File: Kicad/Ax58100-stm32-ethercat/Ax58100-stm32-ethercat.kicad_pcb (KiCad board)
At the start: 2 copper layers, 95.3 x 87.9 mm, 183 parts, among them J1 Step1, J10 5V Power IN, J11 24V Field, J12 DAC, J13 Encoder, J14 In_opt2, J15 STLINK, J16 Serial usart1, J17 In_opt1, J18 Out_opt, J2 Step2, J3 Step3, J4 Step4, J5 THCAD, J6 In1-4, J7 In5-8, J8 Output1-2, J9 Output3-4, SW1 SW PB, U10 AMS1117-1.2, U11 AX58100, U12 TXS0108EPW, U3 MAX3485CSA/ESA, U4 TLP292-4, U5 TLP292-4, U6 TLP292-4, U7 STM32F407VGT6, U8 AMS1117-3.3, U9 24LC32A, Y1 8 MHz, Y2 NXK25.000AE12F-KAB6-12

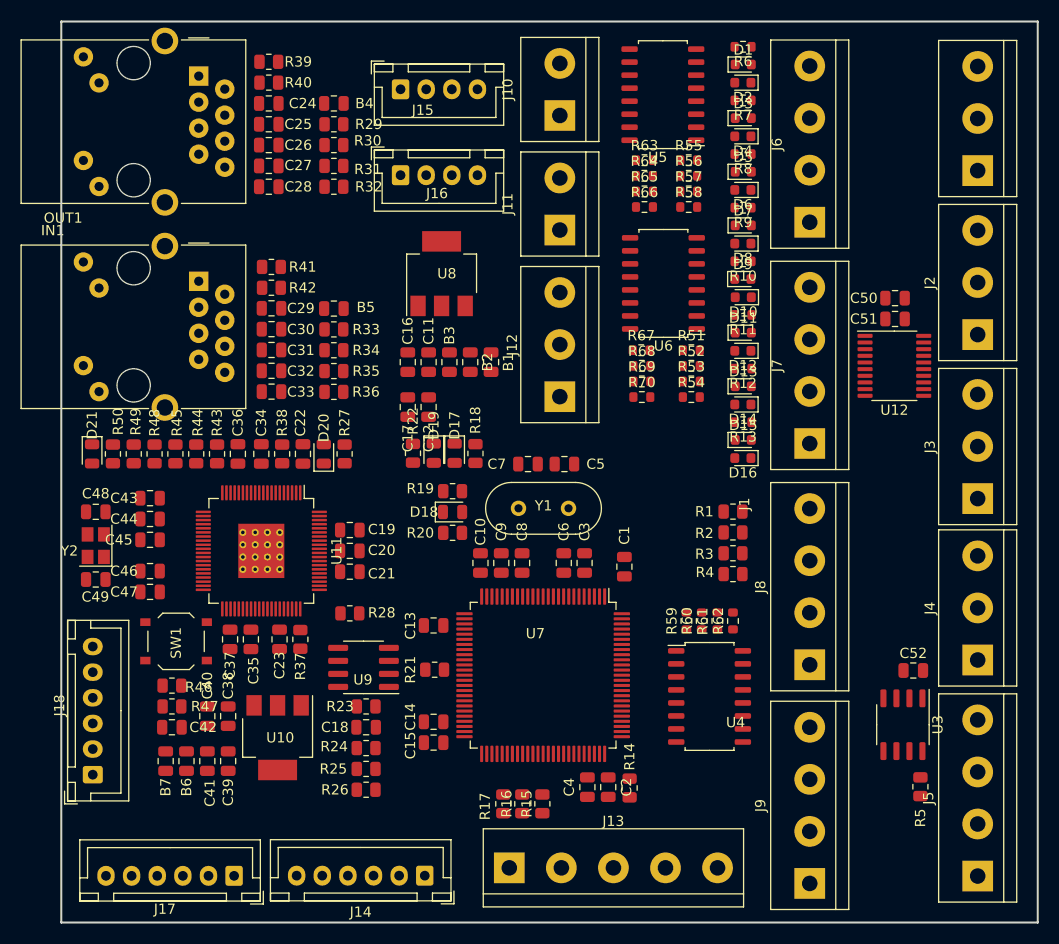
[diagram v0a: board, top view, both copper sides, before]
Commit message: Might be in final shape.
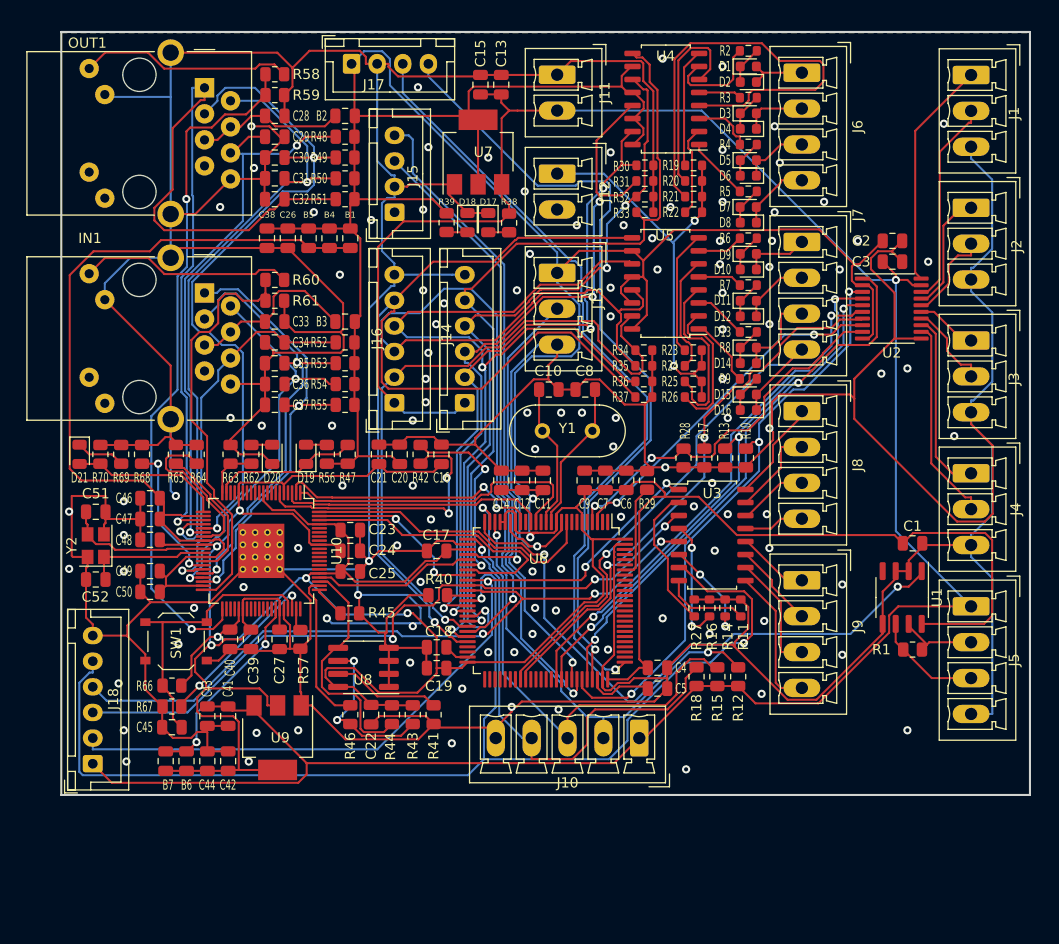
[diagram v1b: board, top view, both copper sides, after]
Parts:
- J1, J2, J3, J4: footprint TerminalBlock:TerminalBlock_bornier-3_P5.08mm -> Connector_Phoenix_MC:PhoenixContact_MCV_1,5_3-G-3.5_1x03_P3.50mm_Vertical
- J10: renamed from J13; footprint TerminalBlock:TerminalBlock_bornier-5_P5.08mm -> Connector_Phoenix_MC:PhoenixContact_MCV_1,5_5-G-3.5_1x05_P3.50mm_Vertical
- J11: renamed from J10; footprint TerminalBlock:TerminalBlock_bornier-2_P5.08mm -> Connector_Phoenix_MC:PhoenixContact_MCV_1,5_2-G-3.5_1x02_P3.50mm_Vertical
- J12: renamed from J11; footprint TerminalBlock:TerminalBlock_bornier-2_P5.08mm -> Connector_Phoenix_MC:PhoenixContact_MCV_1,5_2-G-3.5_1x02_P3.50mm_Vertical
- J13: renamed from J12; footprint TerminalBlock:TerminalBlock_bornier-3_P5.08mm -> Connector_Phoenix_MC:PhoenixContact_MCV_1,5_3-G-3.5_1x03_P3.50mm_Vertical
- J5, J6, J7, J8, J9: footprint TerminalBlock:TerminalBlock_bornier-4_P5.08mm -> Connector_Phoenix_MC:PhoenixContact_MCV_1,5_4-G-3.5_1x04_P3.50mm_Vertical
- R10: renamed from R1; value 4.7k -> 4k7
- R13: renamed from R2; value 4.7k -> 4k7
- R17: renamed from R3; value 4.7k -> 4k7
- R2: renamed from R6; value 1k -> 4k7
- R28: renamed from R4; value 4.7k -> 4k7
- R3: renamed from R7; value 1k -> 4k7
- R4: renamed from R8; value 1k -> 4k7
- R5: renamed from R9; value 1k -> 4k7
- R6: renamed from R10; value 1k -> 4k7
- R7: renamed from R11; value 1k -> 4k7
- R8: renamed from R12; value 1k -> 4k7
- R9: renamed from R13; value 1k -> 4k7
- moved J14 51.3 mm to (125.5, 86.2), turned to 90 degrees
- moved J16 46.2 mm to (118.6, 86.2), turned to 90 degrees
- moved R56 44.0 mm to (112.0, 91.2), turned to 90 degrees
- moved C13 32.2 mm to (129.0, 55.1)
- moved C15 32.2 mm to (127.0, 55.1)
- moved J9 29.6 mm to (158.4, 103.5), turned to -90 degrees
- moved J5 26.3 mm to (174.9, 106.0), turned to -90 degrees
- moved R12 26.1 mm to (152.1, 112.9)
- moved J8 24.8 mm to (158.4, 87.0), turned to -90 degrees
- moved D18 22.7 mm to (125.7, 68.6)
- moved R38 22.7 mm to (129.8, 68.6)
- moved D17 22.7 mm to (127.8, 68.6)
- moved R39 22.7 mm to (123.7, 68.6)
- moved R15 22.7 mm to (150.1, 112.9)
- moved R62 21.1 mm to (104.6, 91.2), turned to 90 degrees
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- renumbered B4 to B2, B5 to B3, B2 to B4, B3 to B5, C52 to C1, C7 to C10, C8 to C11, C9 to C12, C12 to C13, C10 to C14, C17 to C15, C22 to C16, C13 to C17, C14 to C18, C15 to C19, C50 to C2, C34 to C20, C36 to C21, C18 to C22, C19 to C23, C20 to C24, C21 to C25, C11 to C26, C23 to C27, C24 to C28, C25 to C29, C51 to C3, C26 to C30, C27 to C31, C28 to C32, C29 to C33, C30 to C34, C31 to C35, C32 to C36, C33 to C37, C16 to C38, C35 to C39, C2 to C4, C37 to C40, C38 to C41, C39 to C42, C40 to C43, C41 to C44, C42 to C45, C43 to C46, C44 to C47, C45 to C48, C46 to C49, C4 to C5, C47 to C50, C48 to C51, C49 to C52, C1 to C6, C3 to C7, C5 to C8, C6 to C9, D19 to D18, D20 to D19, D18 to D20, J17 to J14, J16 to J15, J14 to J16, J15 to J17, R5 to R1, R62 to R11, R17 to R12, R61 to R14, R16 to R15, R60 to R16, R15 to R18, R55 to R19, R56 to R20, R57 to R21, R58 to R22, R51 to R23, R52 to R24, R53 to R25, R54 to R26, R59 to R27, R19 to R29, R63 to R30, R64 to R31, R65 to R32, R66 to R33, R67 to R34, R68 to R35, R69 to R36, R70 to R37, R18 to R38, R22 to R39, R21 to R40, R26 to R41, R38 to R42, R25 to R43, R24 to R44, R28 to R45, R23 to R46, R27 to R47, R29 to R48, R30 to R49, R31 to R50, R32 to R51, R33 to R52, R34 to R53, R35 to R54, R36 to R55, R14 to R56, R37 to R57, R39 to R58, R40 to R59, R41 to R60, R42 to R61, R20 to R62, R43 to R63, R44 to R64, R45 to R65, R46 to R66, R47 to R67, R48 to R68, R49 to R69, R50 to R70, U3 to U1, U11 to U10, U12 to U2, U4 to U3, U5 to U4, U6 to U5, U7 to U6, U8 to U7, U9 to U8, U10 to U9
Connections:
- J6 pad 1: Net-(D7-A) -> Net-(D1-A)
- J6 pad 2: Net-(D5-A) -> Net-(D3-A)
- J6 pad 3: Net-(D3-A) -> Net-(D5-A)
- J6 pad 4: Net-(D1-A) -> Net-(D7-A)
- J7 pad 1: Net-(D15-A) -> Net-(D10-K)
- J7 pad 2: Net-(D13-A) -> Net-(D11-A)
- J7 pad 3: Net-(D11-A) -> Net-(D13-A)
- J7 pad 4: Net-(D10-K) -> Net-(D15-A)
- R1 pad 1: Net-(J5-Pin_2) -> Net-(J5-Pin_3)
- R1 pad 2: Net-(J5-Pin_3) -> Net-(J5-Pin_2)
- U1 pad 6: Net-(J5-Pin_2) -> Net-(J5-Pin_3)
- U1 pad 7: Net-(J5-Pin_3) -> Net-(J5-Pin_2)
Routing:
- net GND: track 0.00 -> 841.0 mm, vias 0 -> 117
- net +3.3V: track 0.00 -> 463.8 mm, vias 0 -> 5
- net +5V: track 0.00 -> 247.1 mm, vias 0 -> 1
- net IO4: track 0.00 -> 119.2 mm, vias 0 -> 2
- net +1V2: track 0.00 -> 107.8 mm, vias 0 -> 3
- net IO12: track 0.00 -> 102.6 mm, vias 0 -> 1
- net IO10: track 0.00 -> 87.8 mm, vias 0 -> 1
- net +3.3VA: track 0.00 -> 85.2 mm
- net IO11: track 0.00 -> 85.0 mm, vias 0 -> 2
- net P1_TXOP: track 0.00 -> 81.7 mm, vias 0 -> 1
- net SWDIO: track 0.00 -> 78.1 mm, vias 0 -> 1
- net IO8: track 0.00 -> 77.8 mm, vias 0 -> 1
- net IO1: track 0.00 -> 75.6 mm, vias 0 -> 3
- net SWCLK: track 0.00 -> 75.6 mm, vias 0 -> 1
- net IO7: track 0.00 -> 73.7 mm, vias 0 -> 3
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- added copper zone on B.Cu, net GND
- added copper zone on F.Cu, net GND
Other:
- board size 95.3 x 87.9 mm -> 94.5 x 74.4 mm
